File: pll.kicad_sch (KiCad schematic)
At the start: 2 parts, among them CN11 UE75-A20-6000T, CN12 U77-A1114-30L1

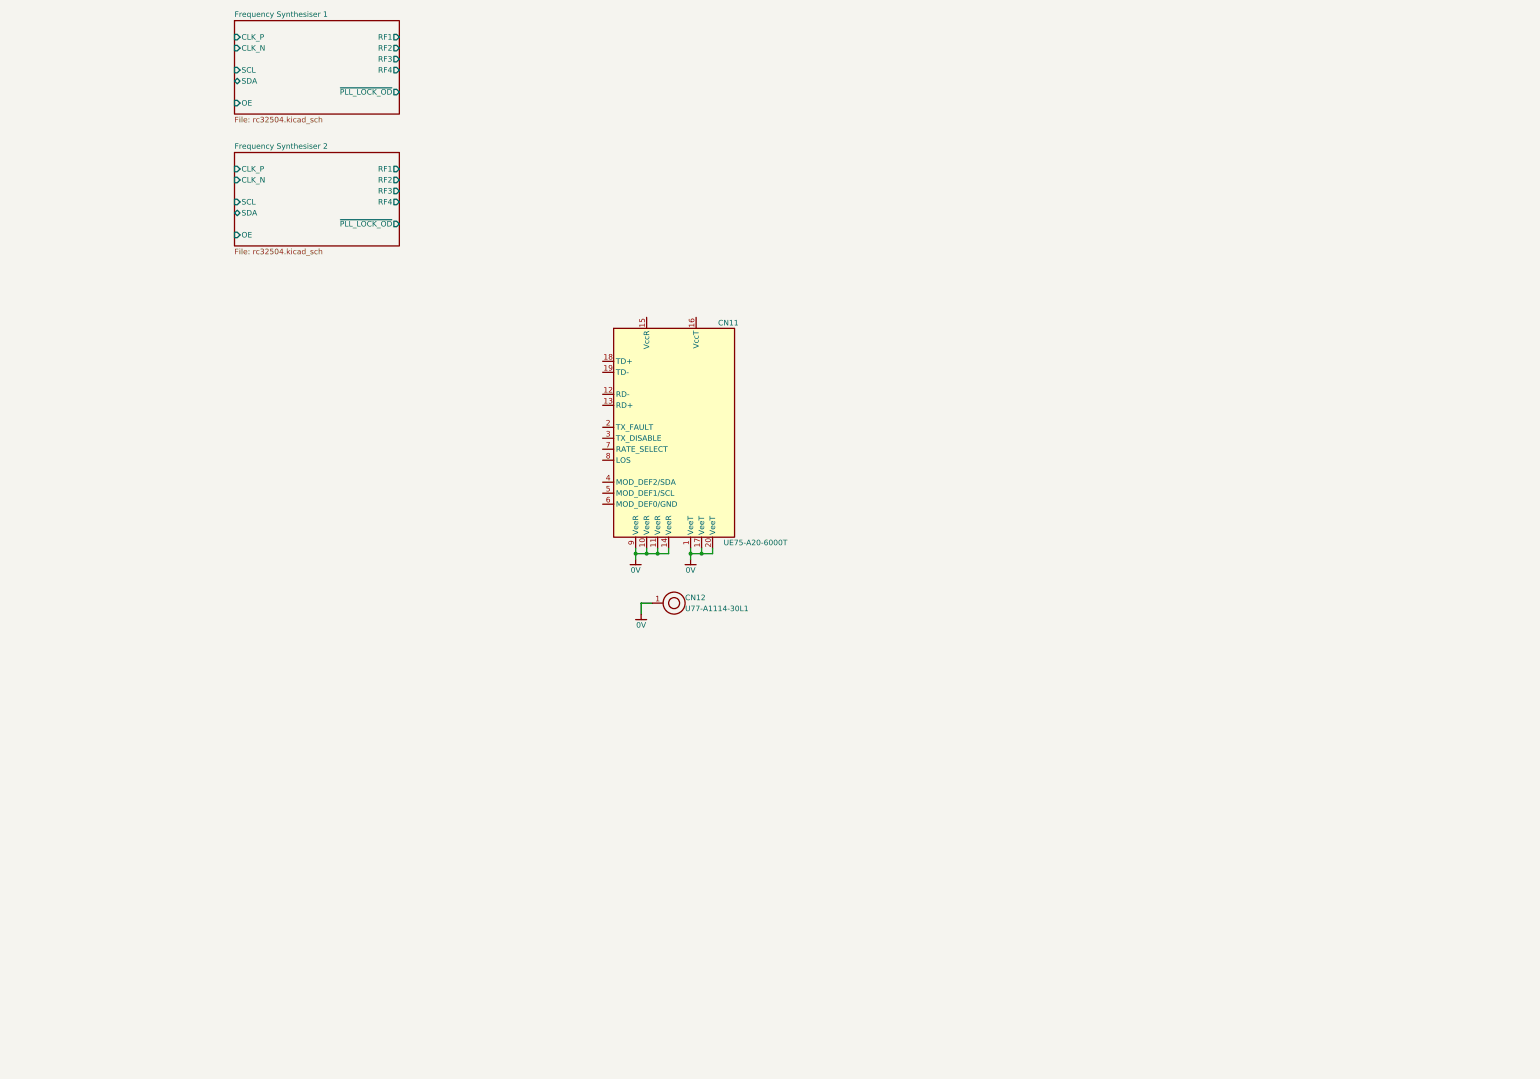
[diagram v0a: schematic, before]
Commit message: Schematic mostly done
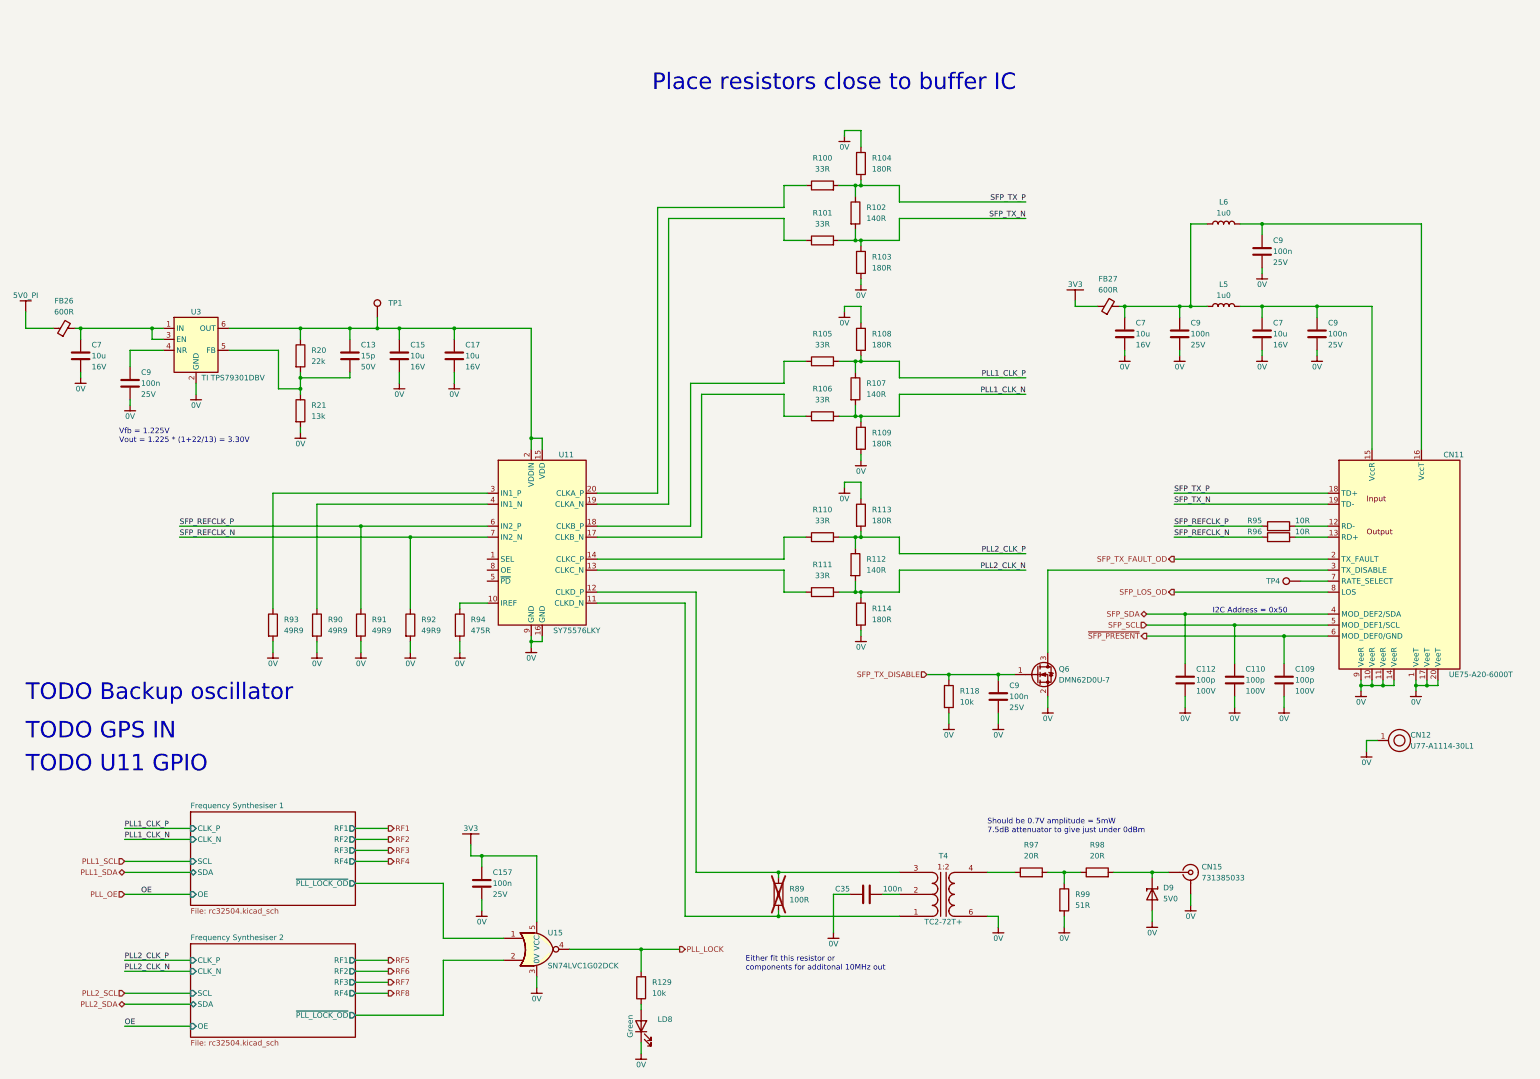
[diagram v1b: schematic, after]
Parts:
- added C109, C110, C112: 100p, Capacitor_SMD:C_0402_1005Metric, symbol Auto_Library_WUT:Kemet C0402C101F1GACTU
- added C13: 15p, Capacitor_SMD:C_0402_1005Metric, symbol Auto_Library_WUT:Kemet C0402C150D5GACTU
- added C15, C17, C7 (x3): 10u, Capacitor_SMD:C_0603_1608Metric, symbol Auto_Library_WUT:Samsung Electro-Mechanics CL10A106MO8NQNC
- added C157, C35, C9 (x5): 100n, Capacitor_SMD:C_0402_1005Metric, symbol Auto_Library_WUT:Yageo CC0402KRX7R8BB104
- added CN15: 731385033, Connector_WUT:BNC_Molex_731385033, symbol Connector_WUT:BNC_Molex_731385033
- added D9: 5V0, Diode_SMD:D_SOD-523, symbol Auto_Library_WUT:Littelfuse AQ3522-01LTG
- added FB26, FB27: 600R, Inductor_SMD:L_0603_1608Metric, symbol Auto_Library_WUT:Murata BLM18AG601SN1D
- added L5, L6: 1u0, Inductor_SMD:L_0603_1608Metric, symbol Auto_Library_WUT:Coilcraft 0603AF-102XJR
- added LD8: Green, LED_SMD:LED_0603_1608Metric, symbol Auto_Library_WUT:Ekinglux_E6C0603VGAC1UDA
- added Q6: DMN62D0U-7, Package_TO_SOT_SMD:SOT-23, symbol FET_WUT:DMN62D0U-7
- added R100, R101, R105, R106, R110, R111: 33R, Resistor_SMD:R_0402_1005Metric, symbol Auto_Library_WUT:KOA Speer RK73H1ETTP33R0F
- added R102, R107, R112: 140R, Resistor_SMD:R_0402_1005Metric, symbol Auto_Library_WUT:KOA Speer RK73H1ETTP1400F
- added R103, R104, R108, R109, R113, R114: 180R, Resistor_SMD:R_0402_1005Metric, symbol Auto_Library_WUT:KOA Speer RK73H1ETTP1800F
- added R118, R129: 10k, Resistor_SMD:R_0402_1005Metric, symbol Auto_Library_WUT:KOA Speer RK73H1ETTP1002F
- added R20: 22k, Resistor_SMD:R_0402_1005Metric, symbol Auto_Library_WUT:KOA Speer RK73H1ETTP2202F
- added R21: 13k, Resistor_SMD:R_0402_1005Metric, symbol Auto_Library_WUT:KOA Speer RK73H1ETTP1302F
- added R89: 100R, Resistor_SMD:R_0402_1005Metric, symbol Auto_Library_WUT:KOA Speer RK73H1ETTP1000F
- added R90, R91, R92, R93: 49R9, Resistor_SMD:R_0402_1005Metric, symbol Auto_Library_WUT:KOA Speer RK73H1ETTP49R9F
- added R94: 475R, Resistor_SMD:R_0402_1005Metric, symbol Auto_Library_WUT:KOA Speer RK73H1ETTP4750F
- added R95, R96: 10R, Resistor_SMD:R_0402_1005Metric, symbol Auto_Library_WUT:KOA Speer RK73H1ETTP10R0F
- added R97, R98: 20R, Resistor_SMD:R_0402_1005Metric, symbol Auto_Library_WUT:KOA Speer RK73H1ETTP20R0F
- added R99: 51R, Resistor_SMD:R_0402_1005Metric, symbol Auto_Library_WUT:KOA Speer RK73H1ETTP51R0F
- added T4: TC2-72T+, RF_WUT:MiniCircuits_AT1521, symbol Transformer_WUT:Minicircuits_TC2-72T
- added TP1, TP4: ~, TestPoint:TestPoint_Pad_D1.0mm, symbol Layout_WUT:TestPoint_1mm_SMD
- added U11: SY75576LKY, Package_SO:TSSOP-20_4.4x6.5mm_P0.65mm, symbol IC_WUT:Microchip_SY75576LKY
- added U15: SN74LVC1G02DCK, Package_TO_SOT_SMD:SOT-353_SC-70-5, symbol Logic_WUT:TI_SN74LVC1G02DCKR
- added U3: TI TPS79301DBV, Package_TO_SOT_SMD:SOT-23-6, symbol IC_WUT:TI_TPS79301DBV
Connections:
- net 0V: now also C109.2, C110.2, C112.2, C15.2, C157.2, C17.2, C35.1, C7.2, C7.2, C7.2, C9.2, C9.2, C9.2, C9.2, C9.2, CN15.2 (Ext), D9.2 (A), LD8.1 (K), Q6.2 (S), R103.2, R104.1, R108.1, R109.2, R113.1, R114.2, R118.2, R21.2, R90.2, R91.2, R92.2, R93.2, R94.2, R99.2, T4.6, U11.16 (GND), U11.9 (GND), U15.3 (0V), U3.2 (GND)
- net Frequency Synthesiser 1/~{PLL_LOCK_OD}: now also U15.1
- net Frequency Synthesiser 2/~{PLL_LOCK_OD}: now also U15.2
- net at CN11.12 (RD-): now also R95.2
- net at CN11.13 (RD+): now also R96.2
- net at CN11.15 (VccR): now also C7.1, C9.1, L5.2
- net at CN11.16 (VccT): now also C9.1, L6.2
- net SFP_TX_P: now reaches CN11.18 (TD+)
- net SFP_TX_P: now also R100.2, R102.1, R104.2
- net SFP_TX_N: now reaches CN11.19 (TD-)
- net SFP_TX_N: now also R101.2, R102.2, R103.1
- net SFP_TX_FAULT_OD: now reaches CN11.2 (TX_FAULT)
- net at CN11.3 (TX_DISABLE): now also Q6.3 (D)
- net SFP_SDA: now reaches CN11.4 (MOD_DEF2/SDA)
- net SFP_SDA: now also C112.1
- net SFP_SCL: now reaches CN11.5 (MOD_DEF1/SCL)
- net SFP_SCL: now also C110.1
- net ~{SFP_PRESENT}: now reaches CN11.6 (MOD_DEF0/GND)
- net ~{SFP_PRESENT}: now also C109.1
- net at CN11.7 (RATE_SELECT): now also TP4.1
- net SFP_LOS_OD: now reaches CN11.8 (LOS)
- new net: R110.1, U11.14 (CLKC_P)
- new net: C35.2, T4.2
- new net: C13.1, C15.1, C17.1, R20.1, TP1.1, U11.15 (VDD), U11.2 (VDDIN), U3.6 (OUT)
- new net: LD8.2 (A), R129.1
- new net: R93.1, U11.3 (IN1_P)
- new net: C7.1, FB26.2, U3.1 (IN), U3.3 (EN)
- new net: R94.1, U11.10 (IREF)
- new net: R89.2, T4.1, U11.11 (CLKD_N)
- new net: R89.1, T4.3, U11.12 (CLKD_P)
- new net: R111.1, U11.13 (CLKC_N)
- new net: R106.1, U11.17 (CLKB_N)
- new net: R105.1, U11.18 (CLKB_P)
- new net: R101.1, U11.19 (CLKA_N)
- new net: R100.1, U11.20 (CLKA_P)
- new net: R90.1, U11.4 (IN1_N)
- new net: R97.1, T4.4
- new net: C7.1, C9.1, FB27.2, L5.1, L6.1
- new net: C13.2, R20.2, R21.1, U3.5 (FB)
- new net: CN15.1 (In), D9.1 (K), R98.2
- new net: R97.2, R98.1, R99.1
- new net: C9.1, U3.4 (NR)
- new net 3V3: C157.1, FB27.1, U15.5 (VCC)
- new net 5V0_PI: FB26.1
- new net PLL1_CLK_N: R106.2, R107.2, R109.1
- new net PLL1_CLK_P: R105.2, R107.1, R108.2
- new net PLL2_CLK_N: R111.2, R112.2, R114.1
- new net PLL2_CLK_P: R110.2, R112.1, R113.2
- new net PLL_LOCK: R129.2, U15.4
- new net SFP_REFCLK_N: R92.1, R96.1, U11.7 (IN2_N)
- new net SFP_REFCLK_P: R91.1, R95.1, U11.6 (IN2_P)
- new net SFP_TX_DISABLE: C9.1, Q6.1 (G), R118.1
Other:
- note added: "Either fit this resistor or components for additonal 10MHz out"
- note added: "I2C Address = 0x50"
- note added: "Place resistors close to buffer IC"
- note added: "Should be 0.7V amplitude = 5mW 7.5dB attenuator to give just under 0dBm"
- note added: "TODO Backup oscillator"
- note added: "TODO GPS IN"
- note added: "TODO U11 GPIO"
- note added: "Vfb = 1.225V Vout = 1.225 * (1+22/13) = 3.30V"
- moved on the sheet: CN12
